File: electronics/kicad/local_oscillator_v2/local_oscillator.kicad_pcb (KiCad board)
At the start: 2 copper layers, 22 parts, among them P1 TestPoint:TestPoint_Pad_1.5x1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, P2 TestPoint:TestPoint_Pad_1.5x1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, P3 TestPoint:TestPoint_Pad_1.5x1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, P4 TestPoint:TestPoint_Pad_1.5x1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, U1 CE3520K3

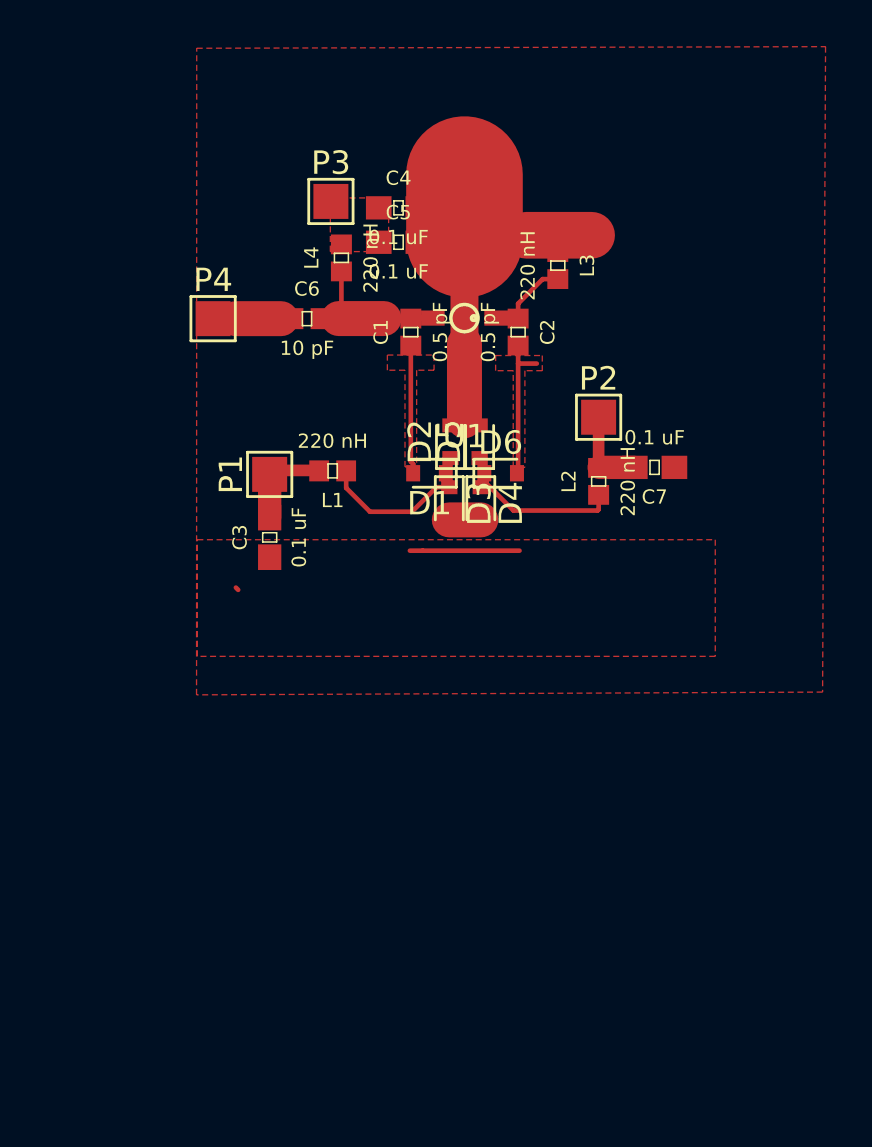
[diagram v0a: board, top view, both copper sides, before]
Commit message: Next rev.
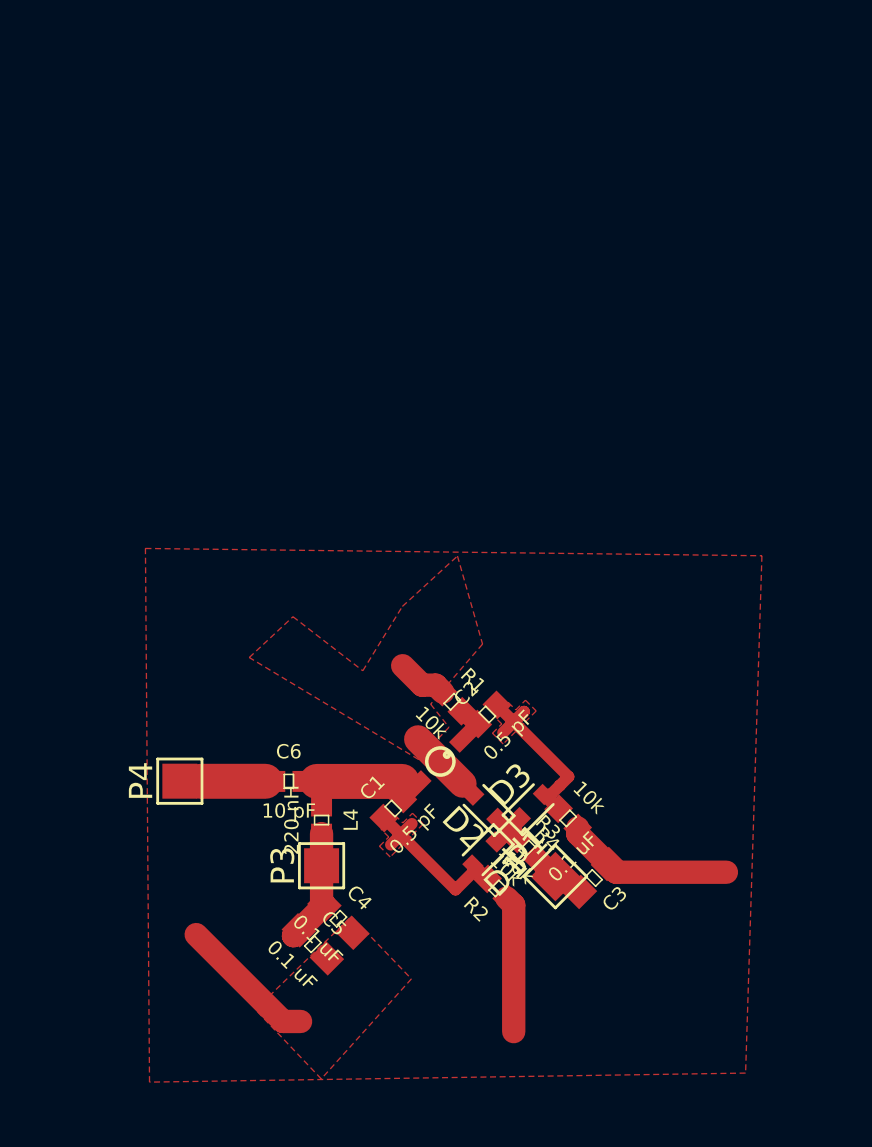
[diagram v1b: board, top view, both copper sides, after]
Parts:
- removed C7: 0.1 uF, Capacitors:0603
- removed D4, D5, D6: D_Capacitance, Diode_SMD:D_SOD-523
- removed L1, L2, L3: 220 nH, Capacitors:0402
- removed P2: TestPoint:TestPoint_Pad_1.5x1.5mm, TestPoint:TestPoint_Pad_1.5x1.5mm
- added R1: 10k, Capacitors:0402, F.Cu at (75.0, 55.6)
- added R2: 10k, Capacitors:0402, F.Cu at (77.0, 63.6)
- added R3: 10k, Capacitors:0402, F.Cu at (78.2, 61.9)
- added R4: 10k, Capacitors:0402, F.Cu at (80.0, 60.6)
- moved C4 30.6 mm to (70.1, 64.9), turned to 315 degrees
- moved C5 30.3 mm to (69.1, 66.0), turned to 315 degrees
- moved P3 28.5 mm to (69.4, 62.6), turned to 90 degrees
- moved L4 24.1 mm to (69.4, 60.7), turned to 270 degrees
- moved P1 21.1 mm to (79.4, 63.1), turned to 45 degrees
- moved C1 20.4 mm to (72.5, 60.2), turned to 45 degrees
- moved C3 20.2 mm to (81.1, 63.1), turned to 225 degrees
- moved P4 19.9 mm to (63.4, 59.0), turned to 90 degrees
- moved C6 19.9 mm to (68.0, 59.0)
- moved U1 19.0 mm to (74.5, 58.2), turned to 45 degrees
- moved D1 16.5 mm to (76.4, 62.1), turned to 225 degrees
- moved C2 16.4 mm to (76.5, 56.1), turned to 45 degrees
- moved D2 15.7 mm to (76.4, 60.1), turned to 135 degrees
- moved D3 13.4 mm to (78.4, 60.1), turned to 45 degrees
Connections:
- D3 pad 2: Net-(D3-Pad2) -> Net-(C2-Pad2)
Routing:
- net Net-(D4-Pad1): track 7.61 -> 0.00 mm
- net Net-(C4-Pad1): track 0.00 -> 5.31 mm
- net Net-(D1-Pad1): track 7.40 -> 2.73 mm
- net GND: track 19.8 -> 24.1 mm
- net Net-(C3-Pad2): track 4.17 -> 0.00 mm
- net Net-(C2-Pad1): track 3.74 -> 0.00 mm
- net Net-(C7-Pad2): track 3.73 -> 0.00 mm
- net Net-(C1-Pad1): track 5.51 -> 8.02 mm
- net /VCC: track 5.96 -> 3.65 mm
- net Net-(C2-Pad2): track 6.32 -> 8.58 mm
- net Net-(D3-Pad2): track 1.35 -> 0.00 mm
- net Net-(C6-Pad1): track 1.94 -> 3.22 mm
- removed copper zone on F.Cu, net Net-(C4-Pad1)
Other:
- net class Default: trace_width 0.2 -> 1

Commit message: aaa
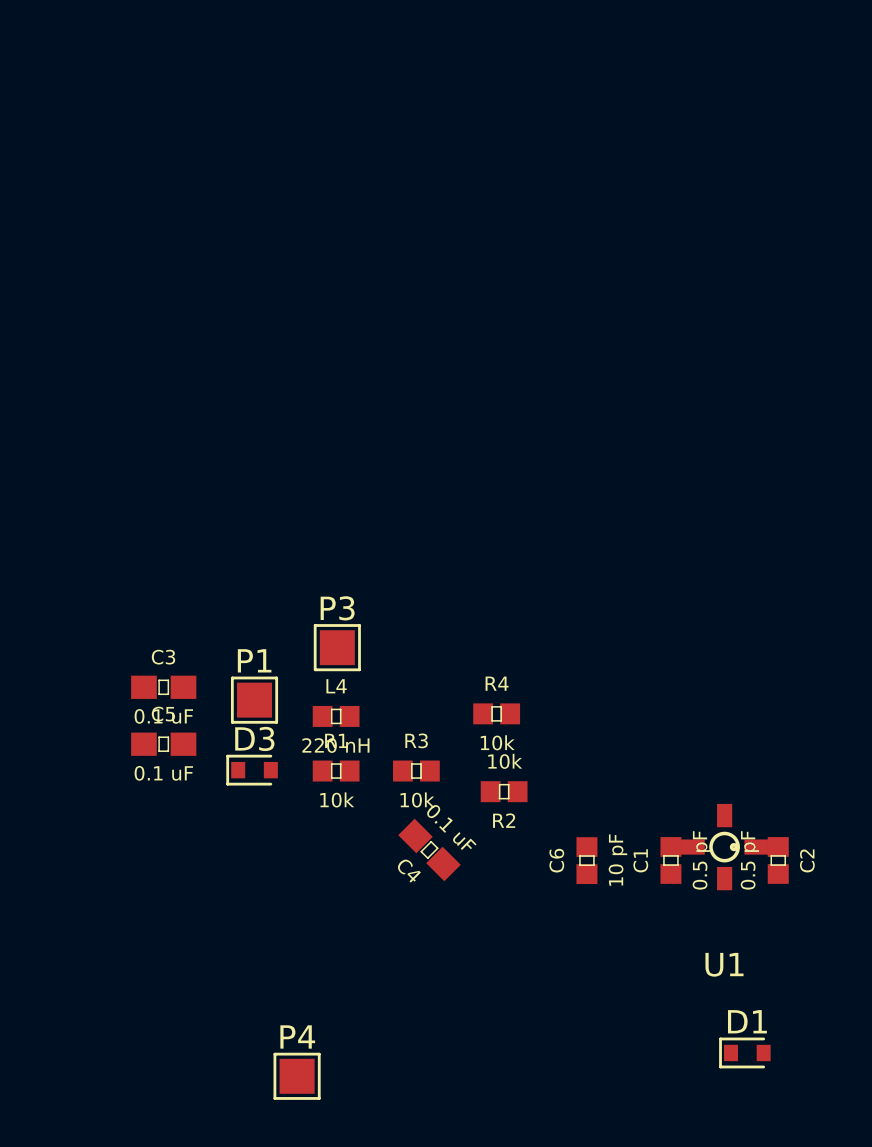
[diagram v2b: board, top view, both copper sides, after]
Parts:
- removed D2: D_Capacitance, Diode_SMD:D_SOD-523
- moved C3 20.2 mm to (62.7, 55.0), turned to 0 degrees
- moved P1 14.9 mm to (66.6, 55.5), turned to 0 degrees
- moved D1 14.1 mm to (87.7, 70.7), turned to 0 degrees
- moved C2 14.0 mm to (89.0, 62.4), turned to 270 degrees
- moved P4 13.6 mm to (68.4, 71.7), turned to 0 degrees
- moved C6 13.2 mm to (80.8, 62.4), turned to 90 degrees
- moved U1 12.7 mm to (86.7, 61.8), turned to 0 degrees
- moved C1 12.1 mm to (84.4, 62.4), turned to 90 degrees
- moved D3 12.0 mm to (66.6, 58.5), turned to 0 degrees
- moved C5 10.7 mm to (62.7, 57.4), turned to 0 degrees
- moved P3 9.37 mm to (70.1, 53.3), turned to 0 degrees
- moved R1 5.80 mm to (70.0, 58.6), turned to 0 degrees
- moved R3 5.80 mm to (73.5, 58.6), turned to 0 degrees
- moved R4 5.43 mm to (76.9, 56.1), turned to 0 degrees
- moved C4 4.89 mm to (74.0, 62.0), turned to 135 degrees
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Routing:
- net GND: track 24.1 -> 0.00 mm
- net Net-(C2-Pad2): track 8.58 -> 0.00 mm
- net Net-(C1-Pad1): track 8.02 -> 0.00 mm
- net Net-(C4-Pad1): track 5.31 -> 0.00 mm
- net /VCC: track 3.65 -> 0.00 mm
- net Net-(C6-Pad1): track 3.22 -> 0.00 mm
- net Net-(D1-Pad1): track 2.73 -> 0.00 mm
- removed copper zone on F.Cu, net GND
- removed copper zone on F.Cu, net Net-(C1-Pad1)
- removed copper zone on F.Cu, net Net-(C2-Pad2)
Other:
- net class Default: trace_width 1 -> 1.5

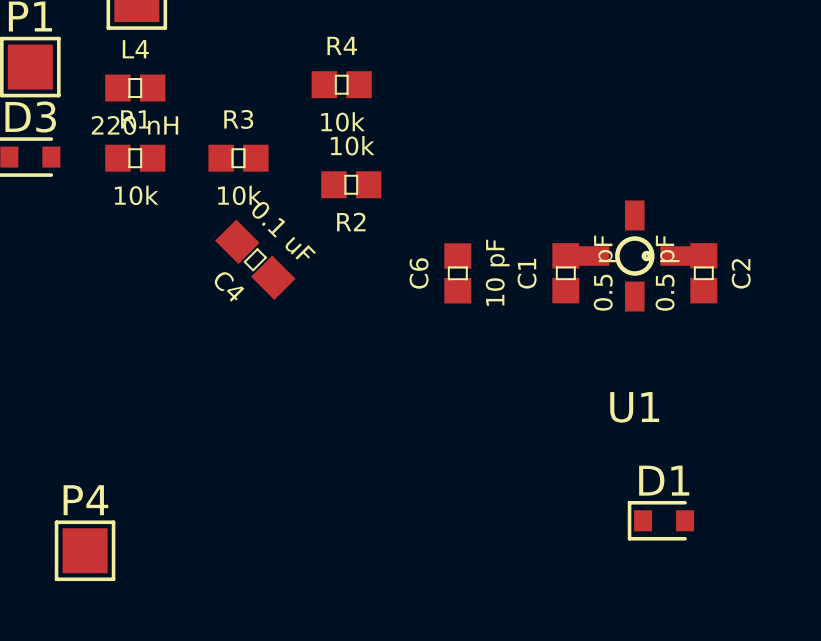
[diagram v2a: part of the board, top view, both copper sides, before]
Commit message: Nephelometer
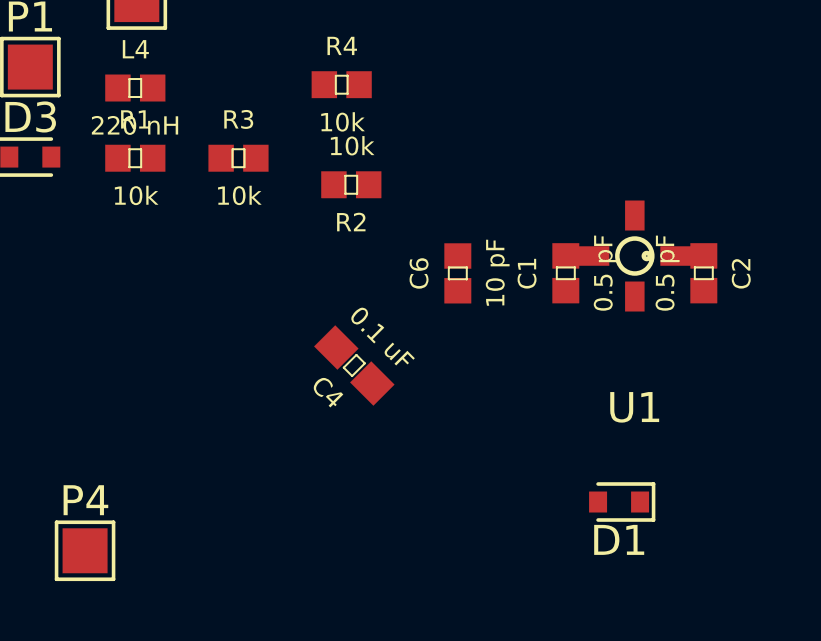
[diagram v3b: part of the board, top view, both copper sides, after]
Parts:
- moved C4 4.83 mm to (77.3, 65.5)
- moved D1 1.62 mm to (86.2, 70.0), turned to 180 degrees
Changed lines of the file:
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@@
   )
   (module Diode_SMD:D_SOD-523 (layer F.Cu)
-    (at 87.675 70.65)
+    (at 86.175 70.025 180)
     (descr "http://www.diodes.com/datasheets/ap02001.pdf p.144")
     (tags "Diode SOD523")
@@
       (effects (font (size 1 1) (thickness 0.15)))
     )
-    (pad 1 smd rect (at -0.7 0 180) (size 0.6 0.7) (layers F.Cu F.Paste F.Mask)
+    (pad 1 smd rect (at -0.7 0) (size 0.6 0.7) (layers F.Cu F.Paste F.Mask)
       (net 8 "Net-(D1-Pad1)"))
-    (pad 2 smd rect (at 0.7 0 180) (size 0.6 0.7) (layers F.Cu F.Paste F.Mask)
+    (pad 2 smd rect (at 0.7 0) (size 0.6 0.7) (layers F.Cu F.Paste F.Mask)
       (net 9 "Net-(C1-Pad1)"))
     (model ${KISYS3DMOD}/Diode_SMD.3dshapes/D_SOD-523.wrl
@@
   )
   (module Capacitors:0603 (layer F.Cu)
-    (at 74.05 61.95 135)
+    (at 77.35 65.475 135)
     (descr "GENERIC 1608 (0603) PACKAGE")
     (tags "GENERIC 1608 (0603) PACKAGE")

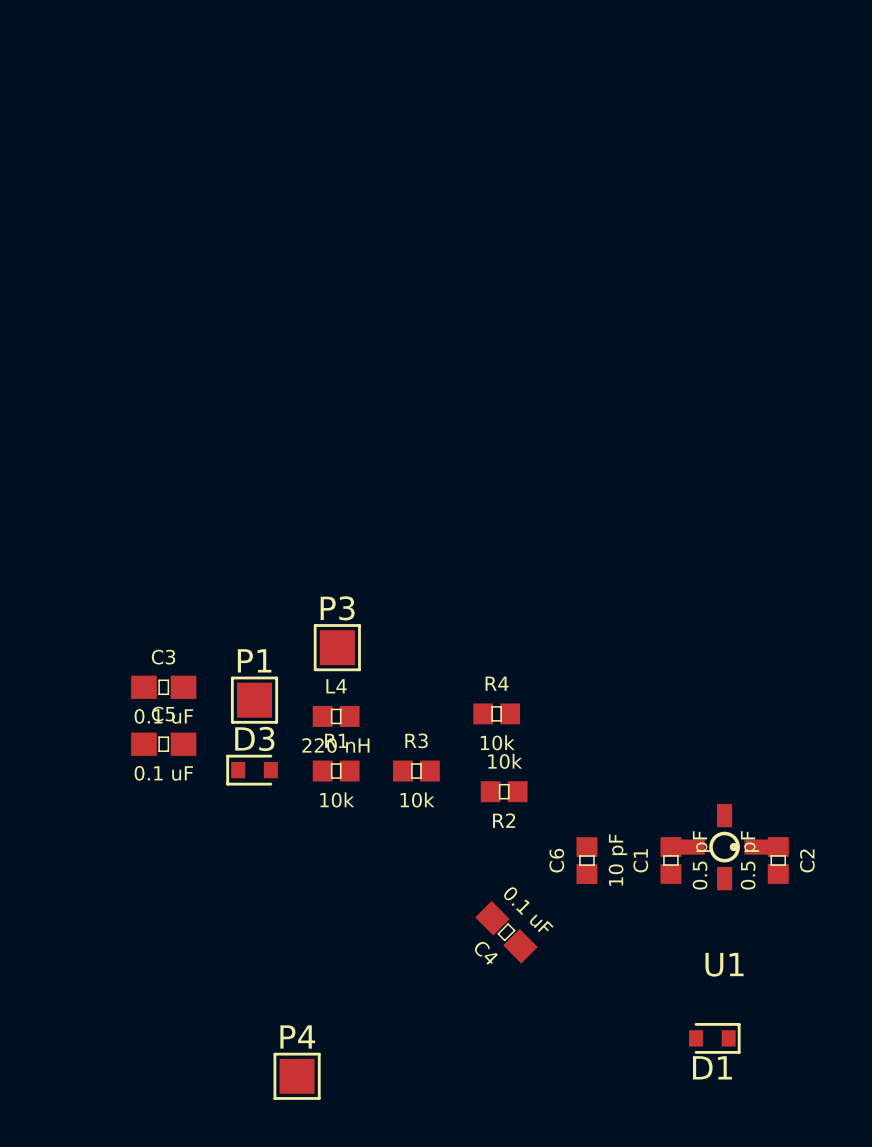
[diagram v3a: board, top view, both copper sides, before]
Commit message: Paper
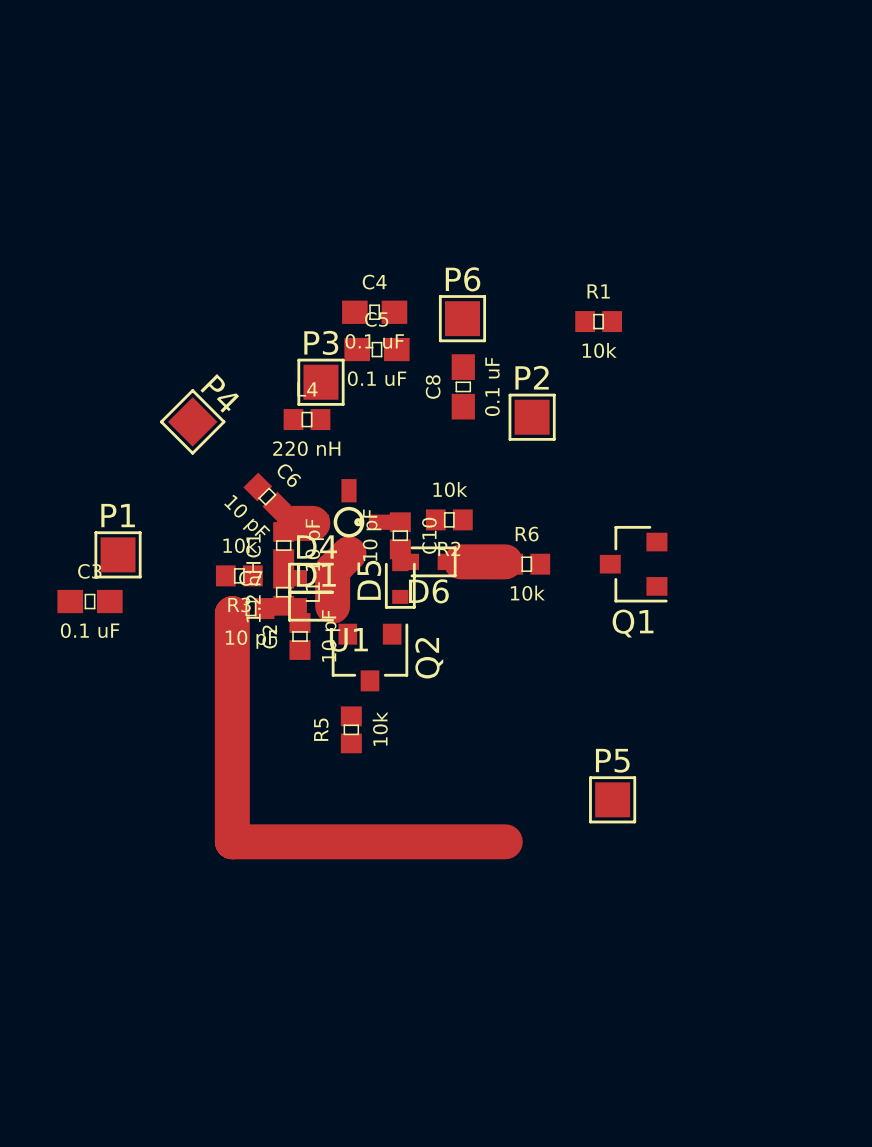
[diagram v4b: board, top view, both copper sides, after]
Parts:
- removed D3: D_Capacitance, Diode_SMD:D_SOD-523
- removed R4: 10k, Capacitors:0402
- added C10: 10 pF, Capacitors:0402, F.Cu at (72.8, 48.5)
- added C7: 10 pF, Capacitors:0402, F.Cu at (66.4, 51.6)
- added C8: 0.1 uF, Capacitors:0603, F.Cu at (75.5, 42.1)
- added D4: D_Capacitance, Diode_SMD:D_SOD-523, F.Cu at (69.2, 50.3)
- added D5: PiN, Diode_SMD:D_SOD-523, F.Cu at (72.8, 50.4)
- added D6: PiN, Diode_SMD:D_SOD-523, F.Cu at (74.0, 49.6)
- added L1: 1.2 nH, Capacitors:0402, F.Cu at (67.8, 50.9)
- added P2: TestPoint:TestPoint_Pad_1.5x1.5mm, TestPoint:TestPoint_Pad_1.5x1.5mm, F.Cu at (78.5, 43.4)
- added P5: TestPoint:TestPoint_Pad_1.5x1.5mm, TestPoint:TestPoint_Pad_1.5x1.5mm, F.Cu at (81.9, 59.8)
- added P6: TestPoint:TestPoint_Pad_1.5x1.5mm, TestPoint:TestPoint_Pad_1.5x1.5mm, F.Cu at (75.5, 39.2)
- added Q1: BSS138, Package_TO_SOT_SMD:SOT-23, F.Cu at (82.8, 49.7)
- added Q2: BSS138, Package_TO_SOT_SMD:SOT-23, F.Cu at (71.5, 53.7)
- added R5: 10k, Capacitors:0402, F.Cu at (70.7, 56.8)
- added R6: 10k, Capacitors:0402, F.Cu at (78.2, 49.7)
- C1, C2: value 0.5 pF -> 10 pF
- moved P4 28.4 mm to (63.9, 43.6), turned to 315 degrees
- moved C4 27.2 mm to (71.7, 38.9), turned to 0 degrees
- moved D1 25.1 mm to (69.2, 51.5), turned to 0 degrees
- moved C2 22.6 mm to (68.5, 52.8), turned to 90 degrees
- moved R1 22.3 mm to (81.3, 39.3)
- moved C1 21.4 mm to (67.8, 48.9)
- moved U1 21.3 mm to (70.6, 47.9)
- moved C6 20.8 mm to (67.1, 46.8), turned to 315 degrees
- moved C5 19.2 mm to (71.8, 40.5)
- moved L4 12.8 mm to (68.8, 43.5)
- moved R2 11.9 mm to (74.9, 47.8)
- moved P3 11.4 mm to (69.4, 41.9)
- moved R3 11.3 mm to (65.9, 50.2), turned to 180 degrees
- moved P1 8.54 mm to (60.7, 49.3)
- moved C3 4.85 mm to (59.5, 51.3)
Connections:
- D1 pad 1: Net-(D1-Pad1) -> Net-(C2-Pad2)
- D1 pad 2: Net-(C1-Pad1) -> GND
- R1 pad 2: Net-(C2-Pad1) -> Net-(C10-Pad1)
- R2 pad 1: GND -> Net-(C8-Pad2)
- R2 pad 2: Net-(C1-Pad1) -> Net-(C10-Pad2)
- R3 pad 1: Net-(D1-Pad1) -> Net-(C2-Pad2)
- U1 pad 4: Net-(C2-Pad1) -> Net-(C10-Pad1)
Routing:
- net Net-(C7-Pad1): track 0.00 -> 23.4 mm
- net GND: track 0.00 -> 2.54 mm
- net /VCC: track 0.00 -> 0.80 mm
